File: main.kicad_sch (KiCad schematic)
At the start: 23 parts, among them U1 LMC555xCMX, U2 LT8374RUFM-WPBF, U3 TPS7B8133QDGNRQ1

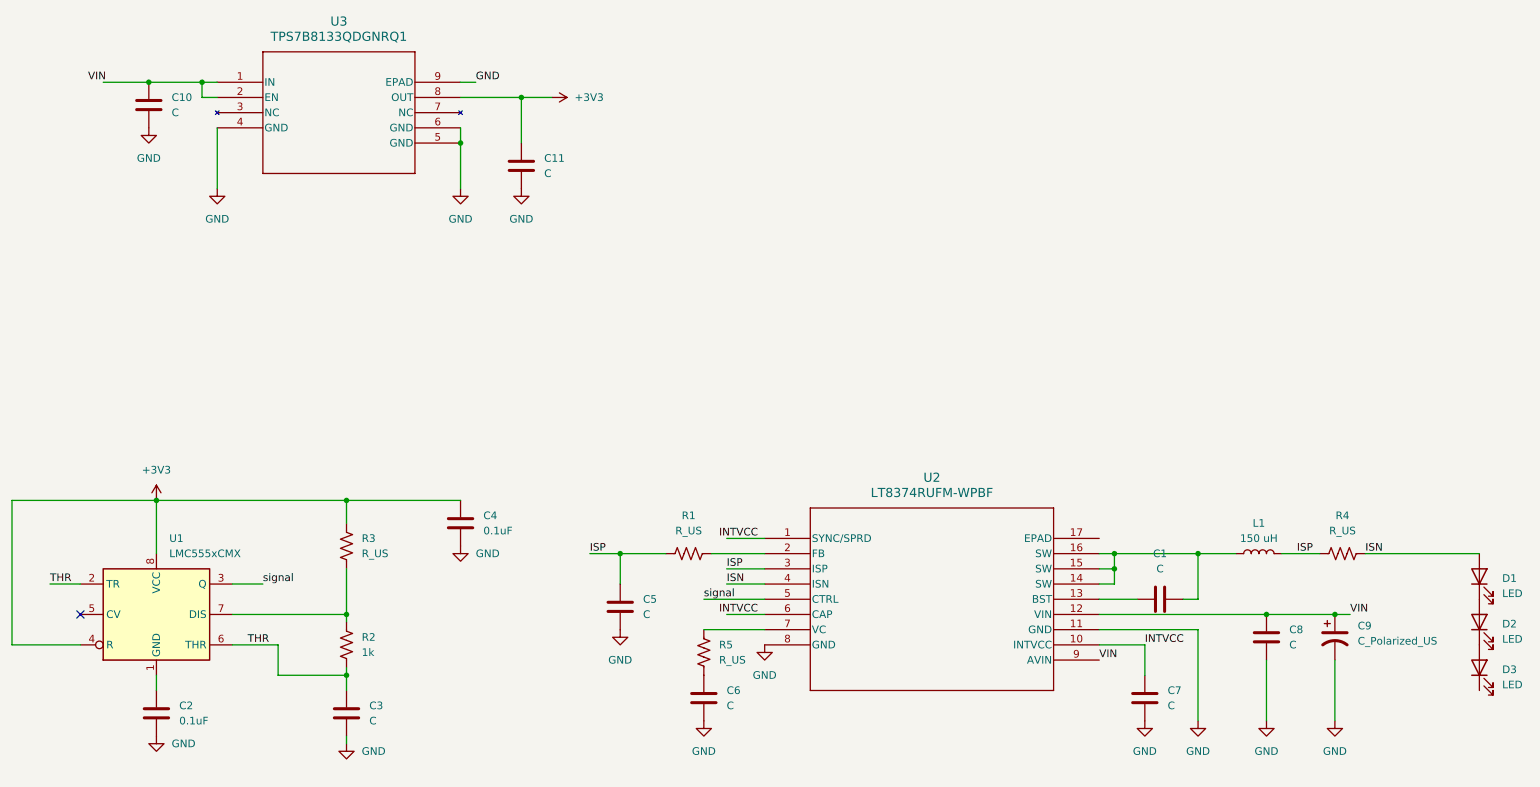
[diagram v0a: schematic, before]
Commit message: values, footprints, and part info complete
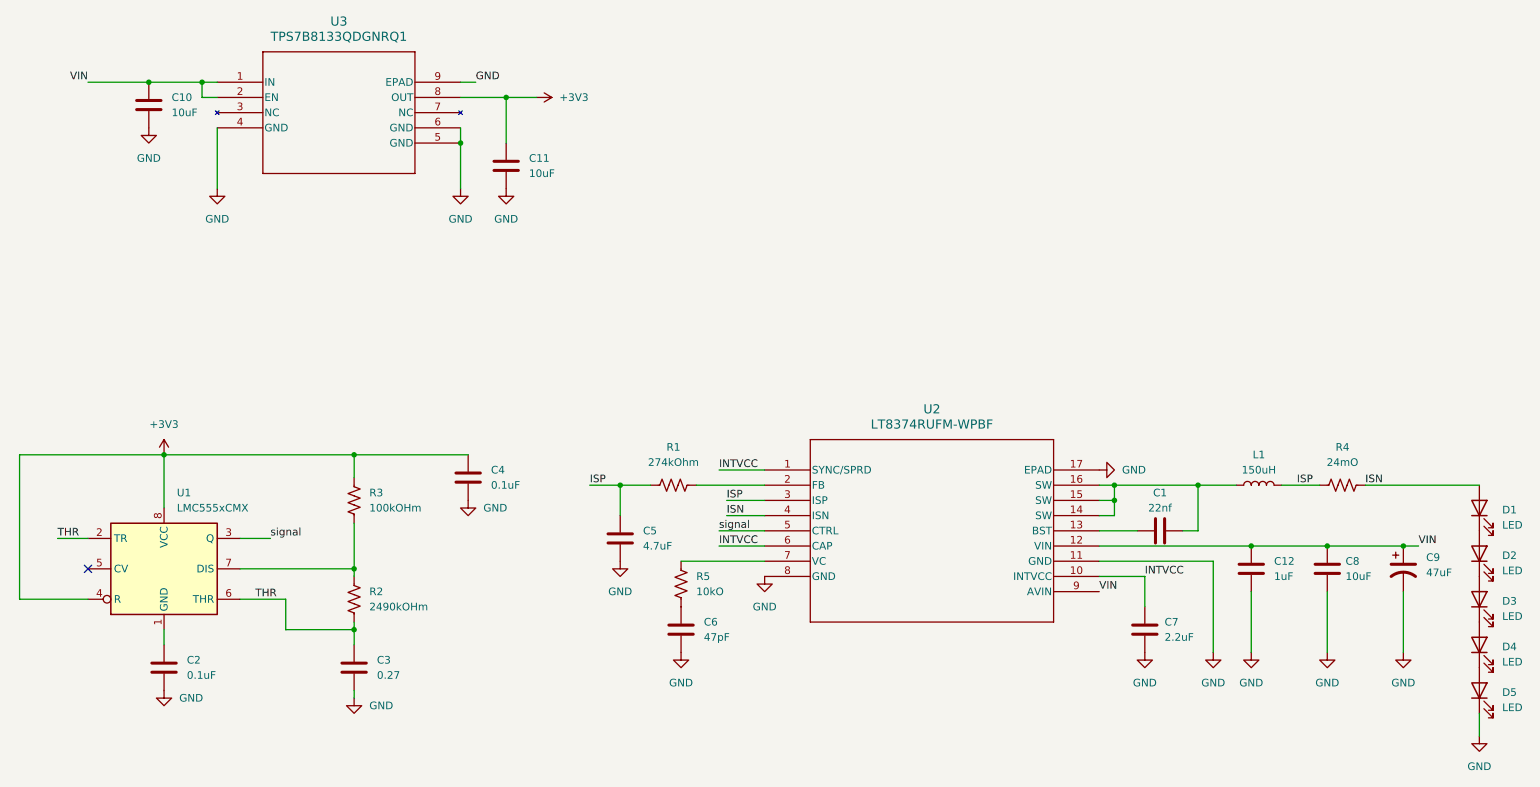
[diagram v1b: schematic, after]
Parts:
- added C12: 1uF, Capacitor_SMD:C_0603_1608Metric, symbol Device:C
- added D4, D5: LED, _NavLights:LED_JB3030AWT_3X3_CRE, symbol Device:LED
- C1: value C -> 22nf; footprint (none) -> Capacitor_SMD:C_0805_2012Metric; Mfr (none) -> Murata Electronics; Mfr P/N (none) -> GCM21B5C1H223FA16L; Supplier_1 (none) -> DigiKey; Supplier_1 P/N (none) -> 490-GCM21B5C1H223FA16LCT-ND; Supplier_1 Price @ Qty (none) -> 1; Supplier_1 Unit Price (none) -> $0.52
- C10, C11, C8: value C -> 10uF; footprint (none) -> Capacitor_SMD:C_0805_2012Metric; Mfr (none) -> Murata Electronics; Mfr P/N (none) -> GRM21BR61H106KE43L; Supplier_1 (none) -> DigiKey; Supplier_1 P/N (none) -> 490-18663-1-ND; Supplier_1 Price @ Qty (none) -> 1; Supplier_1 Unit Price (none) -> $0.28
- C2, C4: footprint (none) -> Capacitor_SMD:C_0603_1608Metric; Mfr (none) -> KEMET; Mfr P/N (none) -> C0603C104K5RACTU; Supplier_1 (none) -> DigiKey; Supplier_1 P/N (none) -> 399-C0603C104K5RACTUCT-ND; Supplier_1 Price @ Qty (none) -> 1; Supplier_1 Unit Price (none) -> $0.08
- C3: value C -> 0.27; footprint (none) -> Capacitor_SMD:C_0805_2012Metric; Mfr (none) -> YAGEO; Mfr P/N (none) -> CC0805KKX7R9BB274; Supplier_1 (none) -> DigiKey; Supplier_1 P/N (none) -> 13-CC0805KKX7R9BB274CT-ND; Supplier_1 Price @ Qty (none) -> 1; Supplier_1 Unit Price (none) -> $0.20
- C5: value C -> 4.7uF; footprint (none) -> Capacitor_SMD:C_0805_2012Metric; Mfr (none) -> Murata Electronics; Mfr P/N (none) -> GRM21BR61H475KE51L; Supplier_1 (none) -> DigiKey; Supplier_1 P/N (none) -> 490-10751-1-ND; Supplier_1 Price @ Qty (none) -> 1; Supplier_1 Unit Price (none) -> $0.19
- C6: value C -> 47pF; footprint (none) -> Capacitor_SMD:C_0603_1608Metric; Mfr (none) -> Vishay Vitramon; Mfr P/N (none) -> VJ0603A470FXACW1BC; Supplier_1 (none) -> DigiKey; Supplier_1 P/N (none) -> 720-VJ0603A470FXACW1BCCT-ND; Supplier_1 Price @ Qty (none) -> 1; Supplier_1 Unit Price (none) -> $0.13
- C7: value C -> 2.2uF; footprint (none) -> Capacitor_SMD:C_0603_1608Metric; Mfr (none) -> Murata Electronics; Mfr P/N (none) -> GRM188R61H225KE11D; Supplier_1 (none) -> DigiKey; Supplier_1 P/N (none) -> 490-10733-1-ND; Supplier_1 Price @ Qty (none) -> 1; Supplier_1 Unit Price (none) -> $0.25
- C9: value C_Polarized_US -> 47uF; footprint (none) -> _NavLights:CAP_EEEFN2A100L; Mfr (none) -> Chemi-Con; Mfr P/N (none) -> HHXC500ARA470MHA0G; Supplier_1 (none) -> DigiKey; Supplier_1 P/N (none) -> 565-HHXC500ARA470MHA0GCT-ND; Supplier_1 Price @ Qty (none) -> 1; Supplier_1 Unit Price (none) -> $1.09
- D1, D2, D3: footprint (none) -> _NavLights:LED_JB3030AWT_3X3_CRE; Supplier_1 (none) -> DigiKey; Supplier_1 P/N (none) -> 2138-JB3030AWT-P-H65EA0000-N0000001CT-ND; Supplier_1 Price @ Qty (none) -> $0.69 for 10; Supplier_1 Unit Price (none) -> $0.10
- L1: value 150 uH -> 150uH; footprint (none) -> _NavLights:IND_BOURNS_SRN1060
- R1: value R_US -> 274kOhm; footprint (none) -> Resistor_SMD:R_0603_1608Metric; Mfr (none) -> Panasonic Electronic Components; Mfr P/N (none) -> ERA-3AEB2743V; Supplier_1 (none) -> DigiKey; Supplier_1 P/N (none) -> P274KDBCT-ND; Supplier_1 Price @ Qty (none) -> 1; Supplier_1 Unit Price (none) -> $0.10
- R2: value 1k -> 2490kOHm; footprint (none) -> Resistor_SMD:R_0603_1608Metric; Mfr (none) -> Stackpole Electronics Inc; Mfr P/N (none) -> RMCF0603FT2M49; Supplier_1 (none) -> DigKey; Supplier_1 P/N (none) -> RMCF0603FT2M49CT-ND; Supplier_1 Price @ Qty (none) -> 1; Supplier_1 Unit Price (none) -> $0.10
- R3: value R_US -> 100kOHm; footprint (none) -> Resistor_SMD:R_0603_1608Metric; Mfr (none) -> Stackpole Electronics Inc; Mfr P/N (none) -> RMCF0603FT100K; Supplier_1 (none) -> DigiKey; Supplier_1 P/N (none) -> RMCF0603FT100KCT-ND; Supplier_1 Price @ Qty (none) -> 1; Supplier_1 Unit Price (none) -> $0.10
- R4: value R_US -> 24mO; footprint (none) -> Resistor_SMD:R_0805_2012Metric; Mfr (none) -> Panasonic Electronic Components; Mfr P/N (none) -> ERJ-6CWDR024V; Supplier_1 (none) -> DigiKey; Supplier_1 P/N (none) -> P124410CT-ND; Supplier_1 Price @ Qty (none) -> 1; Supplier_1 Unit Price (none) -> $0.61
- R5: value R_US -> 10kO; footprint (none) -> Resistor_SMD:R_0603_1608Metric; Mfr (none) -> Panasonic Electronic Components; Mfr P/N (none) -> ERA-3AEB103V; Supplier_1 (none) -> DigiKey; Supplier_1 P/N (none) -> P10KDBCT-ND; Supplier_1 Price @ Qty (none) -> 1; Supplier_1 Unit Price (none) -> $0.10
- U2: Mfr (none) -> Analog Devices Inc.; Mfr P/N (none) -> LT8374RUFM#WPBF; Supplier_1 (none) -> DigiKey; Supplier_1 P/N (none) -> 505-LT8374RUFM#WPBF-ND; Supplier_1 Price @ Qty (none) -> 1; Supplier_1 Unit Price (none) -> $5.34
- U3: Mfr (none) -> Texas Instruments; Mfr P/N (none) -> TPS7B8133QDGNRQ1; Supplier_1 (none) -> DigiKey; Supplier_1 P/N (none) -> 296-TPS7B8133QDGNRQ1CT-ND; Supplier_1 Price @ Qty (none) -> 1; Supplier_1 Unit Price (none) -> $1.60
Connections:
- net GND: now also U2.17 (EPAD), C12.2, D5.1 (K)
- net INTVCC: now also U2.1 (SYNC/SPRD), U2.6 (CAP)
- net VIN: now also C10.1, U3.1 (IN), U3.2 (EN), C12.1
- net at D3.1 (K): now also D4.2 (A)
- new net: D4.1 (K), D5.2 (A)
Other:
- moved on the sheet: C1, C11, C2, C3, C4, C5, C6, C7, C8, C9, D1, L1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
